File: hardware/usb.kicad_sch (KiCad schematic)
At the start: 19 parts, among them J3 USB_C_Receptacle_USB2.0_14P, J4 USB_C_Receptacle_USB2.0_14P, J5 USB_C_Receptacle_USB2.0_14P, U3 ECP5U_12_CABGA256, U6 FT231XQ, U7 TPD2EUSB30A, U8 TPD2EUSB30A, U9 TPD2EUSB30A

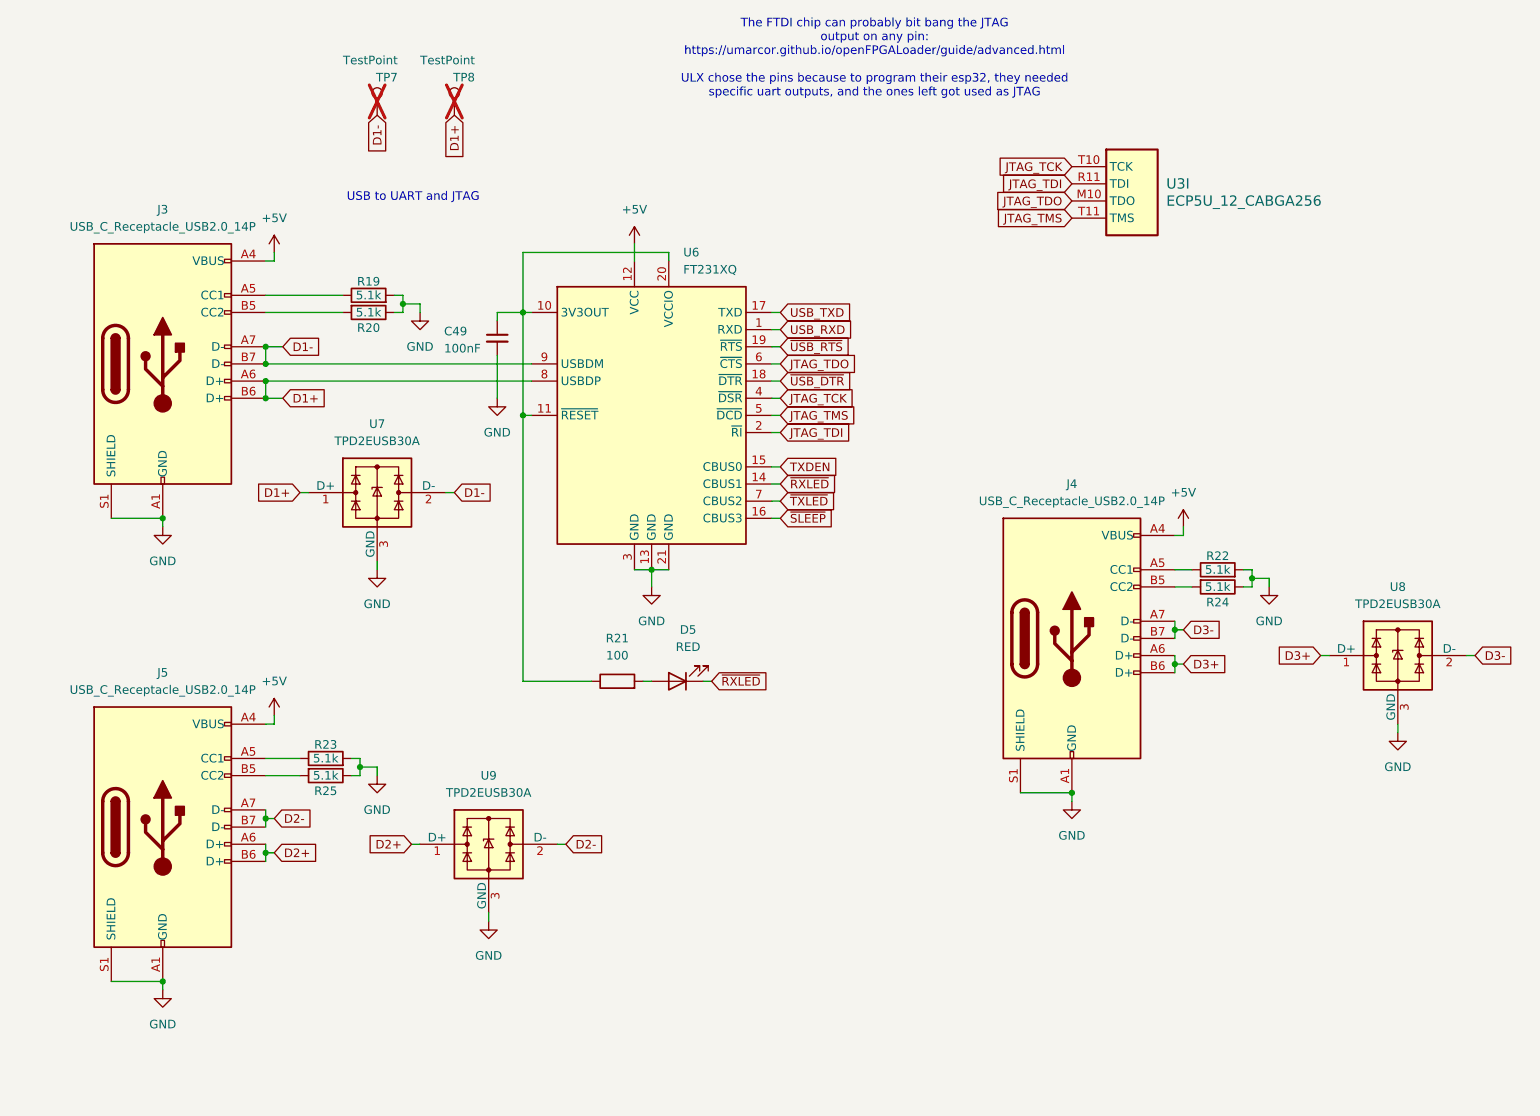
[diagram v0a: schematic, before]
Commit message: Pre-prod fixes
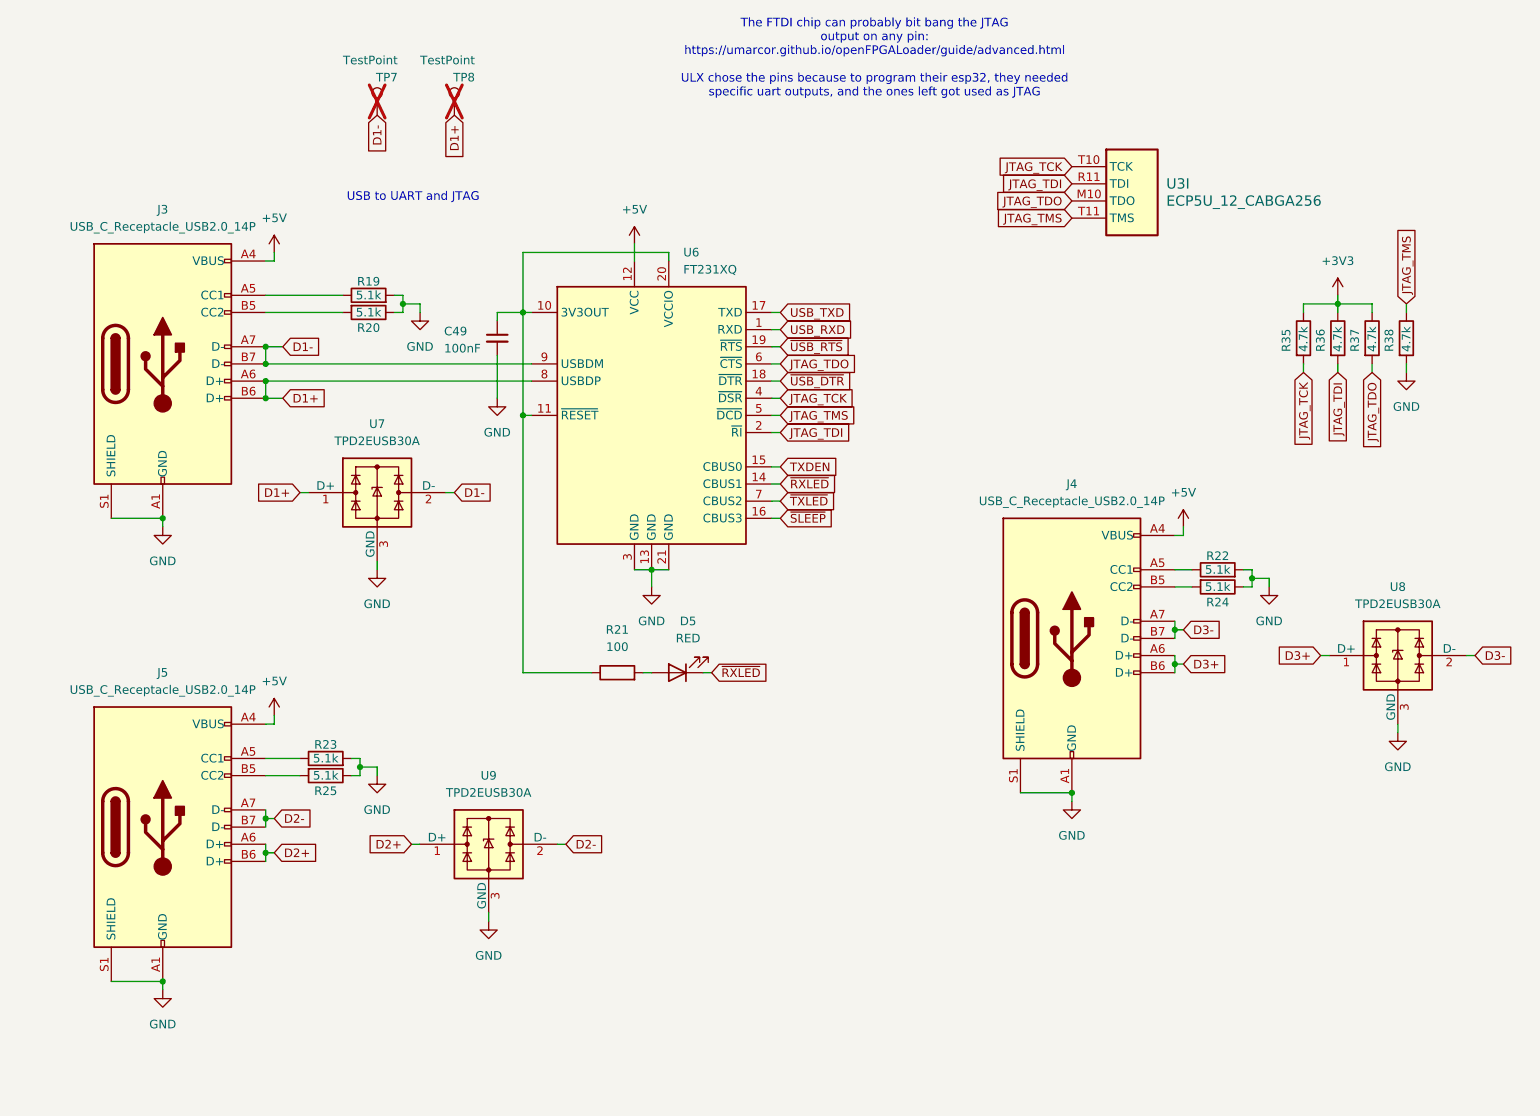
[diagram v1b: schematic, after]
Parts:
- added R35, R36, R37, R38: 4.7k, Resistor_SMD:R_0402_1005Metric, symbol Device:R
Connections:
- net GND: now also R38.2
- net JTAG_TCK: now also R35.2
- net JTAG_TDI: now also R36.2
- net JTAG_TDO: now also R37.2
- net JTAG_TMS: now also R38.1
- new net +3V3: R35.1, R36.1, R37.1
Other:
- moved on the sheet: D5, R21

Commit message: Final revision
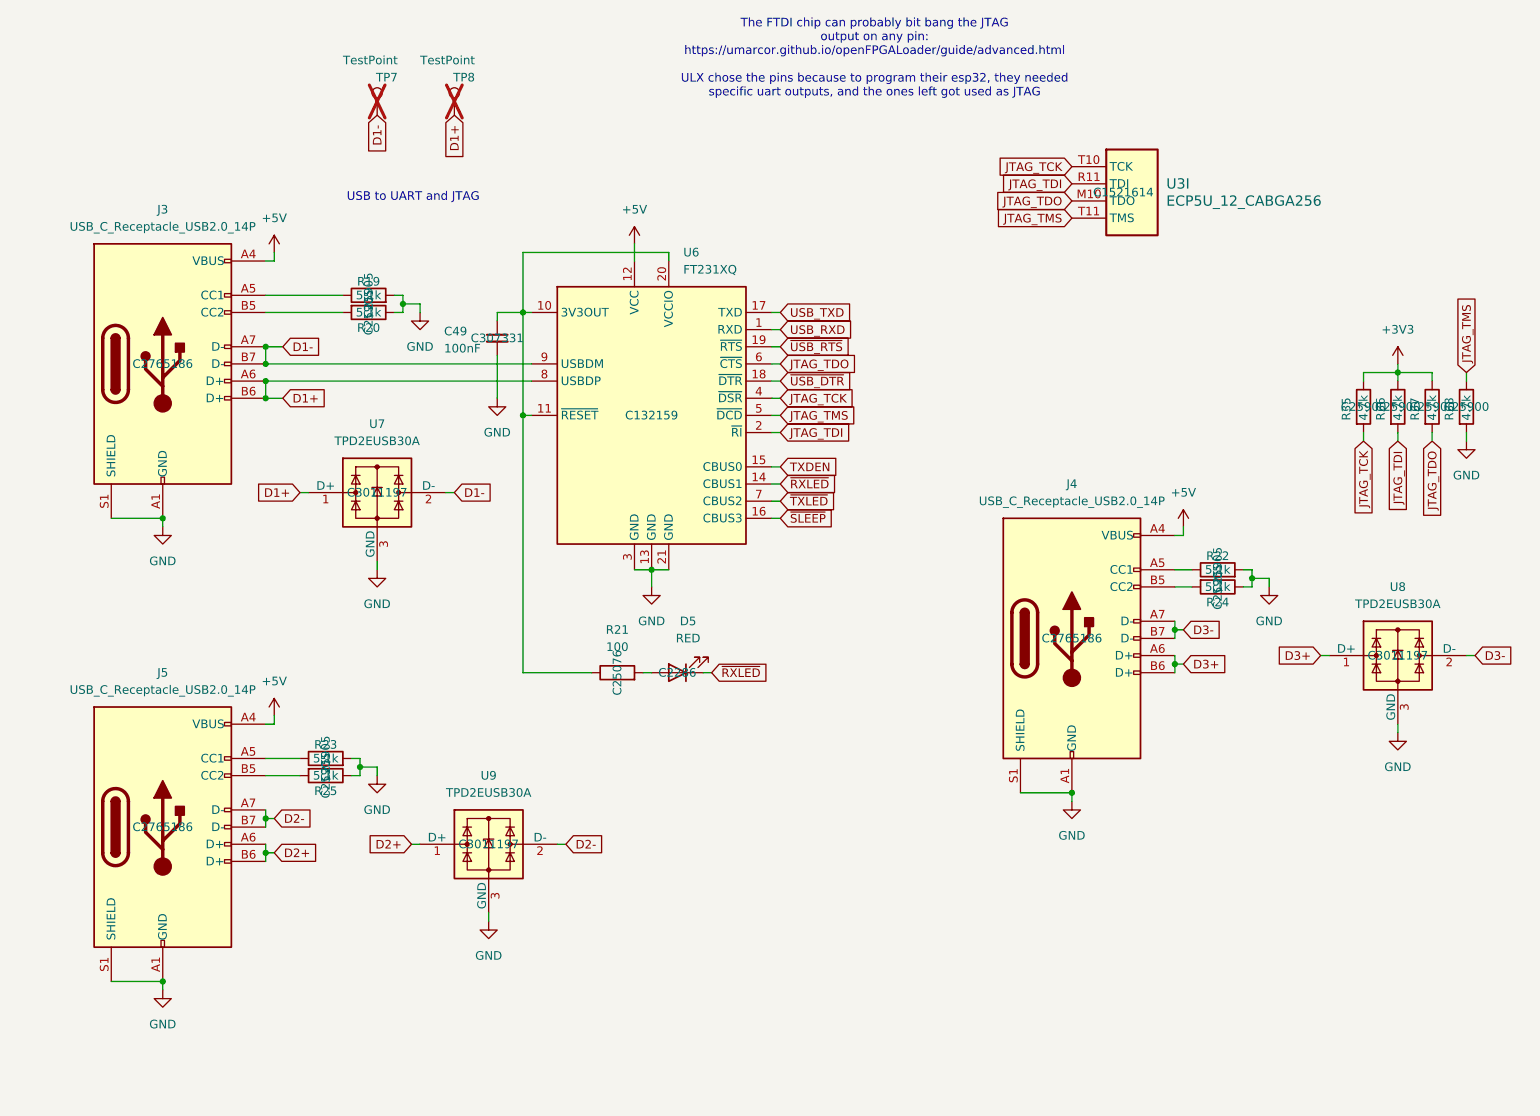
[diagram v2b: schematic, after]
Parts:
- C49: JLCPCB Part # C307331 -> (none); LCSC Part # (none) -> C307331
- D5: JLCPCB Part # C2286 -> (none); LCSC Part # (none) -> C2286
- J3, J4, J5: JLCPCB Part # C2765186 -> (none); LCSC Part # (none) -> C2765186
- R19, R20, R22, R23, R24, R25: JLCPCB Part # C25905 -> (none); LCSC Part # (none) -> C25905
- R21: JLCPCB Part # C25076 -> (none); LCSC Part # (none) -> C25076
- R35, R36, R37, R38: JLCPCB Part # C25900 -> (none); LCSC Part # (none) -> C25900
- U3: JLCPCB Part # C1521614 -> (none); LCSC Part # (none) -> C1521614
- U6: JLCPCB Part # C132159 -> (none); LCSC Part # (none) -> C132159
- U7, U8, U9: JLCPCB Part # C3011197 -> (none); LCSC Part # (none) -> C3011197
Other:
- moved on the sheet: R35, R36, R37, R38

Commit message: Last checks
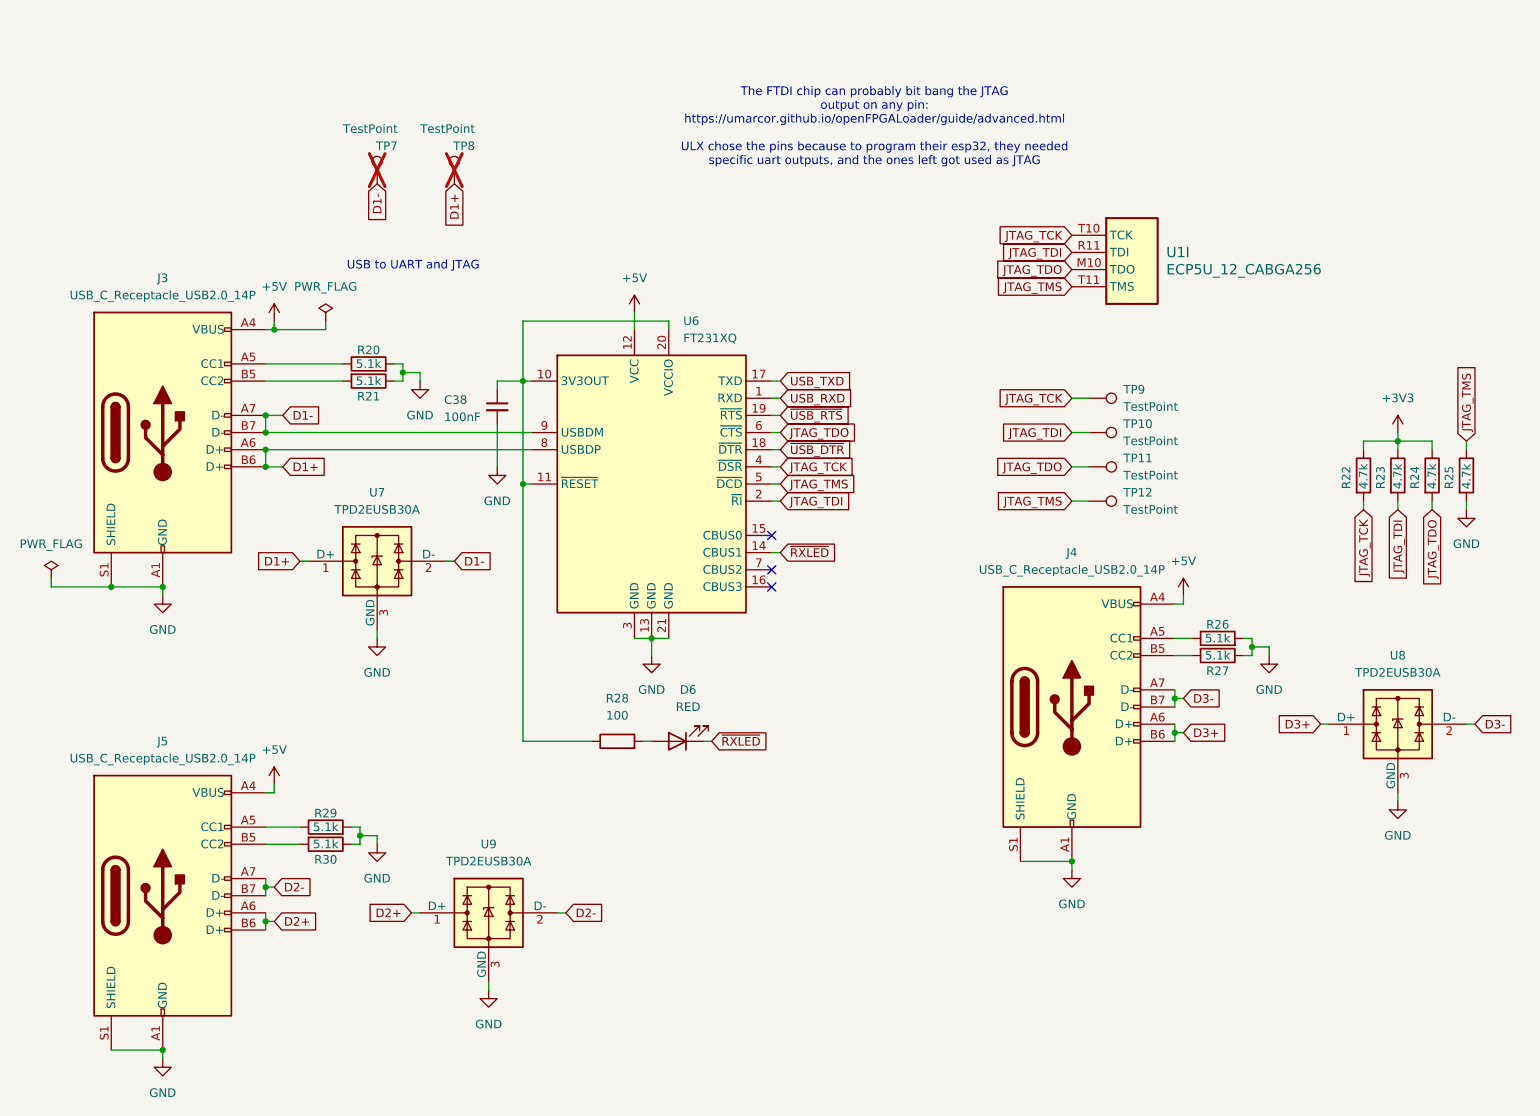
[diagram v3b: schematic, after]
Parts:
- added TP10, TP11, TP12, TP9: TestPoint, TestPoint:TestPoint_Pad_D1.0mm, symbol Connector:TestPoint
- renumbered C49 to C38, D5 to D6, R19 to R20, R20 to R21, R35 to R22, R36 to R23, R37 to R24, R38 to R25, R22 to R26, R24 to R27, R21 to R28, R23 to R29, R25 to R30, U3 to U1
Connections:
- net JTAG_TCK: now also TP9.1
- net JTAG_TDI: now also TP10.1
- net JTAG_TDO: now also TP11.1
- net JTAG_TMS: now also TP12.1
- net TXDEN: no longer names the net of U6.15 (CBUS0)
- net ~{SLEEP}: no longer names the net of U6.16 (CBUS3)
- net ~{TXLED}: no longer names the net of U6.7 (CBUS2)
- no-connect marks 0 -> 3
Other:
- moved on the sheet: C38, D6, J3, J4, J5, R20, R21, R22, R23, R24, R25, R26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
